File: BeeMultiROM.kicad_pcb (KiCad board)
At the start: 2 copper layers, 33.5 x 45 mm, 5 parts, among them SW1 SW_Coded_SH-S3000A, U1 27C128, U2 M27C2001

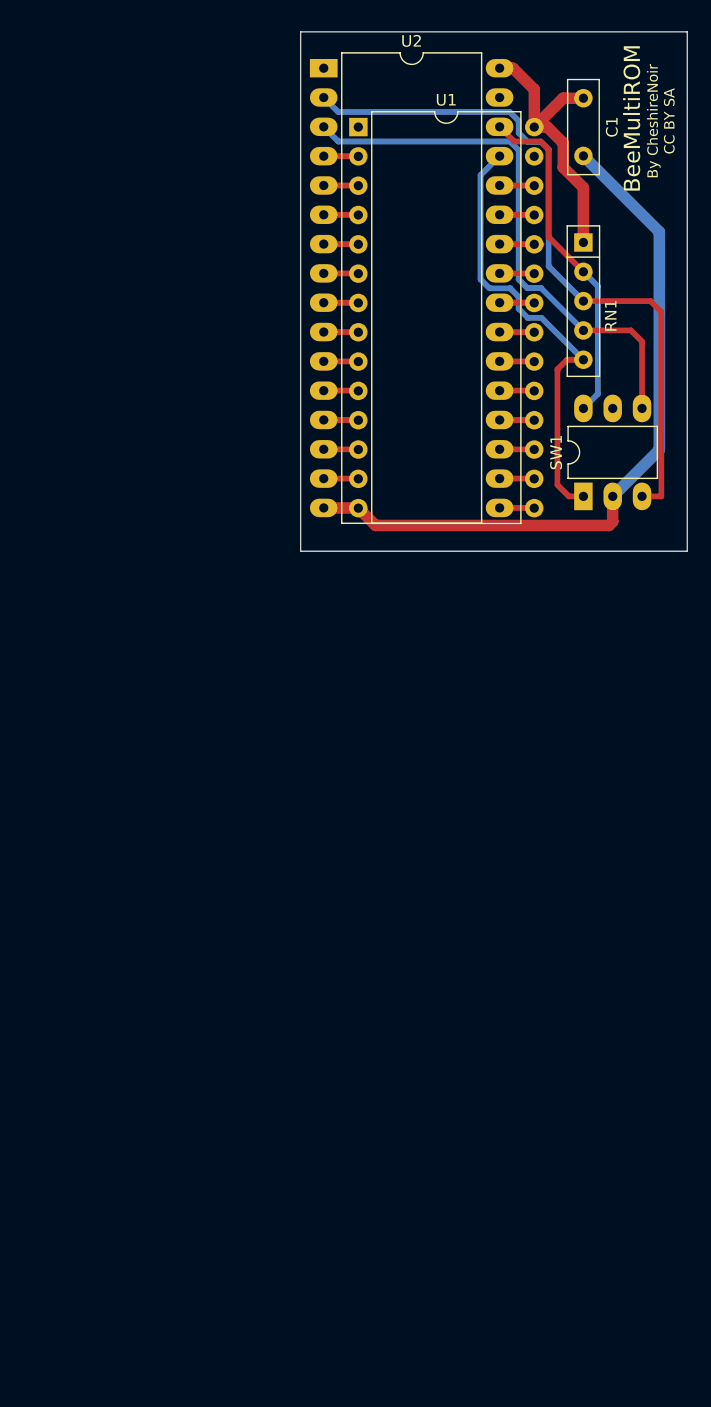
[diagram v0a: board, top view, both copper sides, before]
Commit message: Add files via upload
Super low profile version
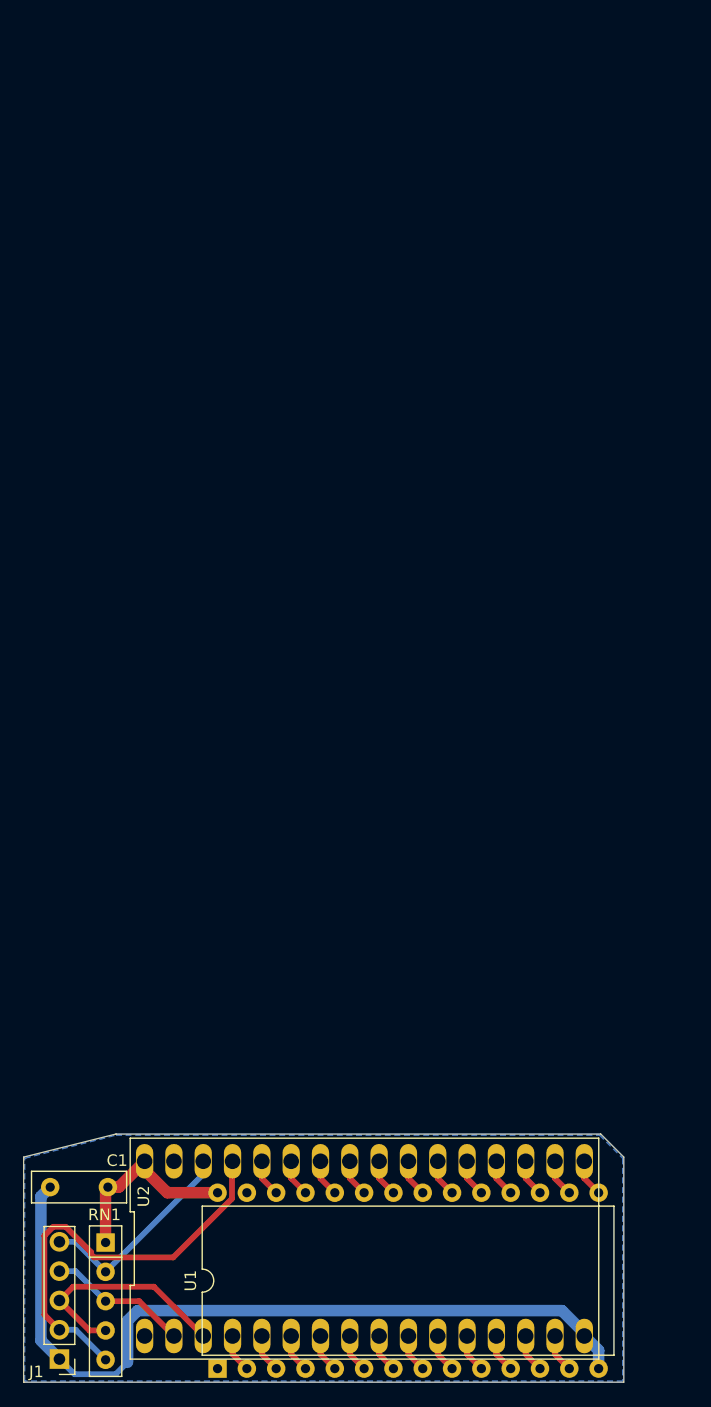
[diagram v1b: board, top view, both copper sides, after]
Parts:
- removed SW1: SW_Coded_SH-S3000A, Package_DIP:DIP-6_W7.62mm_LongPads
- added J1: Conn_01x05, Connector_PinHeader_2.54mm:PinHeader_1x05_P2.54mm_Vertical, F.Cu at (116.1, 139.5)
- U2: footprint Package_DIP:DIP-32_W15.24mm_LongPads -> CheshBits:DIP-32_LP_FATBOY
- moved U1 108.3 mm to (129.8, 140.3), turned to 90 degrees
- moved C1 103.0 mm to (120.3, 124.6), turned to 180 degrees
- moved U2 102.3 mm to (142.5, 129.9)
- moved RN1 96.0 mm to (120.1, 129.4)
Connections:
- U1 pad 1: Net-(U1-Pad1) -> unconnected-(U1-Pad1)
- U1 pad 27: Net-(U1-Pad27) -> unconnected-(U1-Pad27)
- U2 pad 1: Net-(U2-Pad1) -> unconnected-(U2-Pad1)
- U2 pad 31: Net-(U2-Pad31) -> unconnected-(U2-Pad31)
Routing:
- net Net-(J1-Pad4): track 61.1 -> 12.2 mm
- net Net-(J1-Pad3): track 47.6 -> 19.8 mm
- net Net-(J1-Pad5): track 29.9 -> 18.2 mm
- net GND: track 61.9 -> 70.7 mm
- net +5V: track 24.7 -> 16.9 mm
- net Net-(J1-Pad2): track 39.0 -> 36.9 mm
- net Net-(U1-Pad24): track 4.25 -> 3.24 mm
- added copper zone on B.Cu, net GND
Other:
- board size 33.5 x 45 mm -> 52 x 21.5 mm
- net class Default removed
- rule pad_to_mask_clearance: 0.05 -> 0
- board text added: "BeeMultiROM v2.5"
- board text added: "by CheshireNoir CC BY SA"
- board text removed: "BeeMultiROM"
- board text removed: "By CheshireNoir CC BY SA"
